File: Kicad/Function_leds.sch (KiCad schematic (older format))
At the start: 2 parts

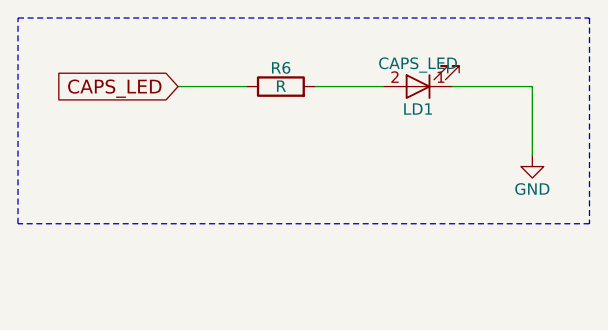
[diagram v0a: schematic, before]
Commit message: - Updated 3 pin header for caps lock
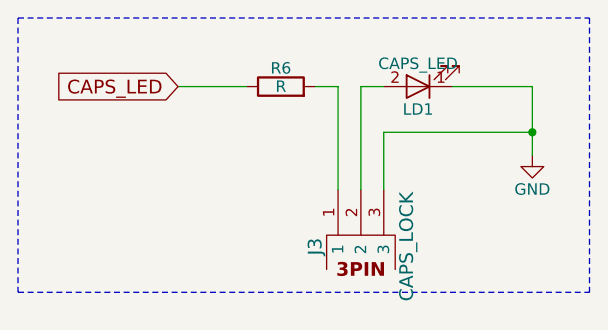
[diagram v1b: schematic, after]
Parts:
- added J3: CAPS_LOCK, Pin_Headers:Pin_Header_Angled_1x03, symbol 3PIN
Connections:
- net GND: now also J3.3
- net at LD1.2 (A): now also J3.2; no longer R6.2
- new net: J3.1, R6.2
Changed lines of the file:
@@
 	1600 1400 1900 1400
-Wire Wire Line
-	2200 1400 2500 1400
 Wire Wire Line
 	2800 1400 3150 1400
@@
 	900  1100 3400 1100
 Wire Notes Line
-	3400 1100 3400 2000
+	3400 1100 3400 2300
 Wire Notes Line
-	3400 2000 900  2000
+	900  1100 900  2300
+$Comp
+L 3PIN J3
+U 1 1 594A7AA3
+P 2400 2050
+F 0 "J3" H 2350 2250 60  0000 C CNN
+F 1 "CAPS_LOCK" H 2350 1850 60  0000 C CNN
+F 2 "Pin_Headers:Pin_Header_Angled_1x03" H 2400 2050 60  0001 C CNN
+F 3 "" H 2400 2050 60  0000 C CNN
+	1    2400 2050
+	0    -1   -1   0
+$EndComp
+Wire Wire Line
+	3150 1600 2500 1600
+Wire Wire Line
+	2500 1600 2500 1850
+Connection ~ 3150 1600
+Wire Wire Line
+	2500 1400 2400 1400
+Wire Wire Line
+	2400 1400 2400 1850
+Wire Wire Line
+	2200 1400 2300 1400
+Wire Wire Line
+	2300 1400 2300 1850
 Wire Notes Line
-	900  2000 900  1100
+	900  2300 3400 2300
 $EndSCHEMATC

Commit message: - First draw for Rev. B
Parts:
- J3: footprint Pin_Headers:Pin_Header_Angled_1x03 -> Pin_Headers:Pin_Header_Angled_1x03_Pitch2.54mm
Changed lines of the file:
@@
 F 0 "J3" H 2350 2250 60  0000 C CNN
 F 1 "CAPS_LOCK" H 2350 1850 60  0000 C CNN
-F 2 "Pin_Headers:Pin_Header_Angled_1x03" H 2400 2050 60  0001 C CNN
+F 2 "Pin_Headers:Pin_Header_Angled_1x03_Pitch2.54mm" H 2400 2050 60  0001 C CNN
 F 3 "" H 2400 2050 60  0000 C CNN
 	1    2400 2050
